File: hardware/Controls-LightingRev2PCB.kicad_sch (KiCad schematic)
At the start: 37 parts, among them IC2 AP2205-W5-7, IC3 ACS724LLCTR-05AU-T, IC4 ACS724LLCTR-05AU-T, IC6 ACS724LLCTR-05AU-T, J1 53307-2471, J3 Conn_02x05_Top_Bottom, J4 Conn_01x02, J5 Conn_01x02, J6 Conn_01x03, Q3 IRLML0030, Q5 IRLML0030, U5 SN74LV1T34DBV

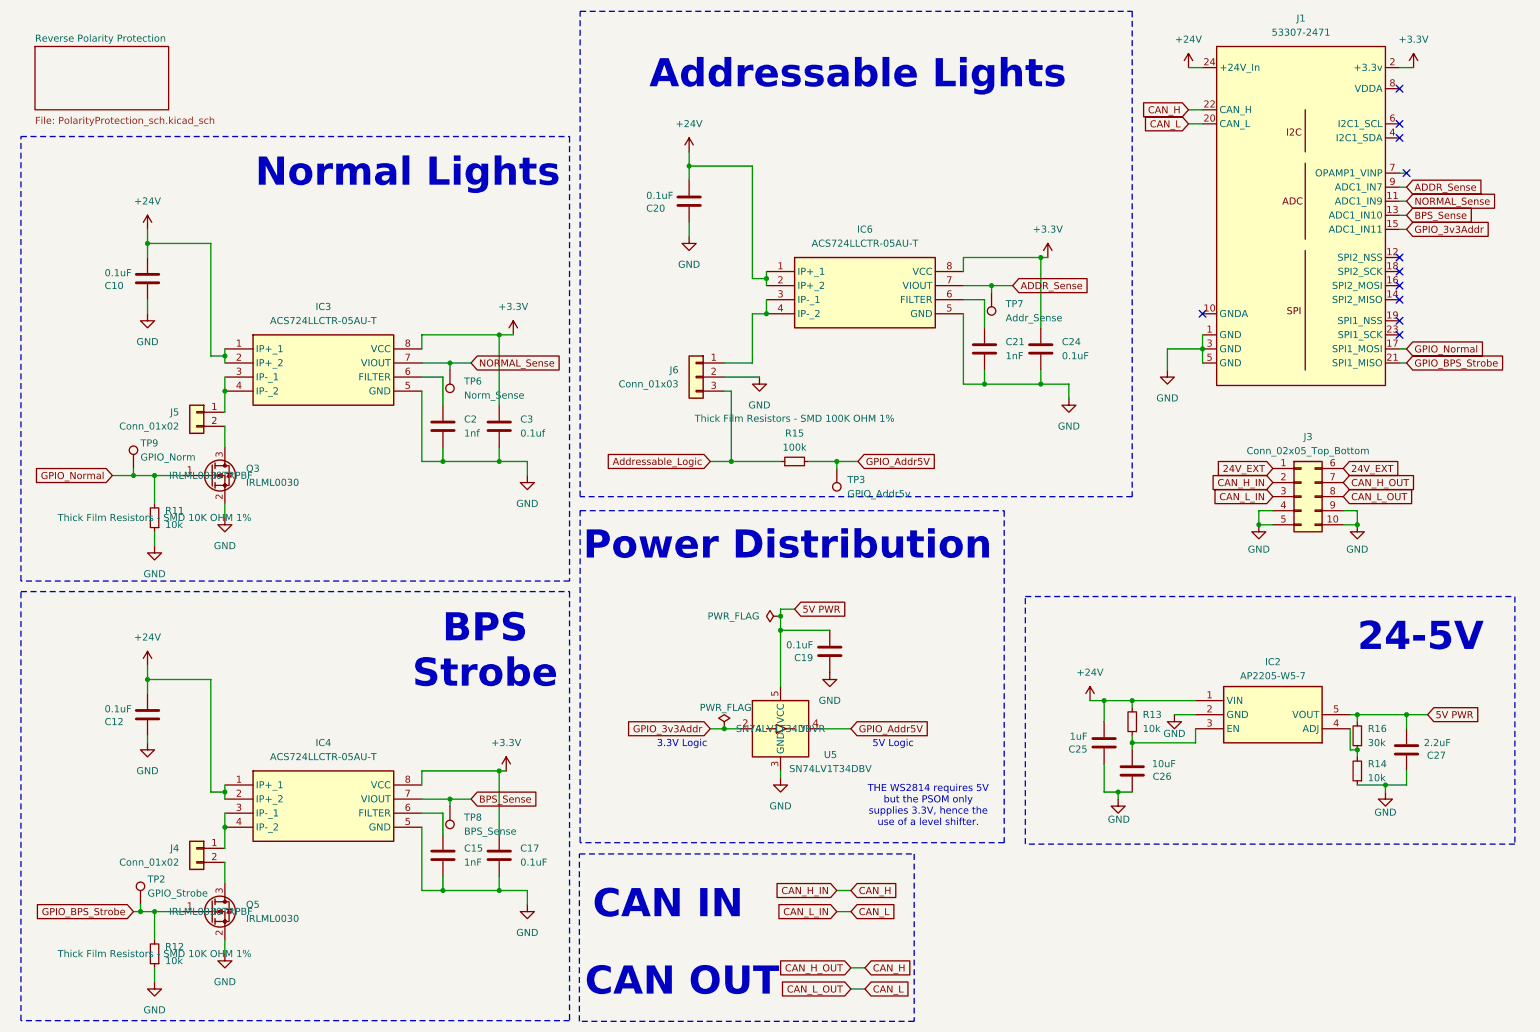
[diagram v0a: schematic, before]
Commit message: Bom and Final Layout
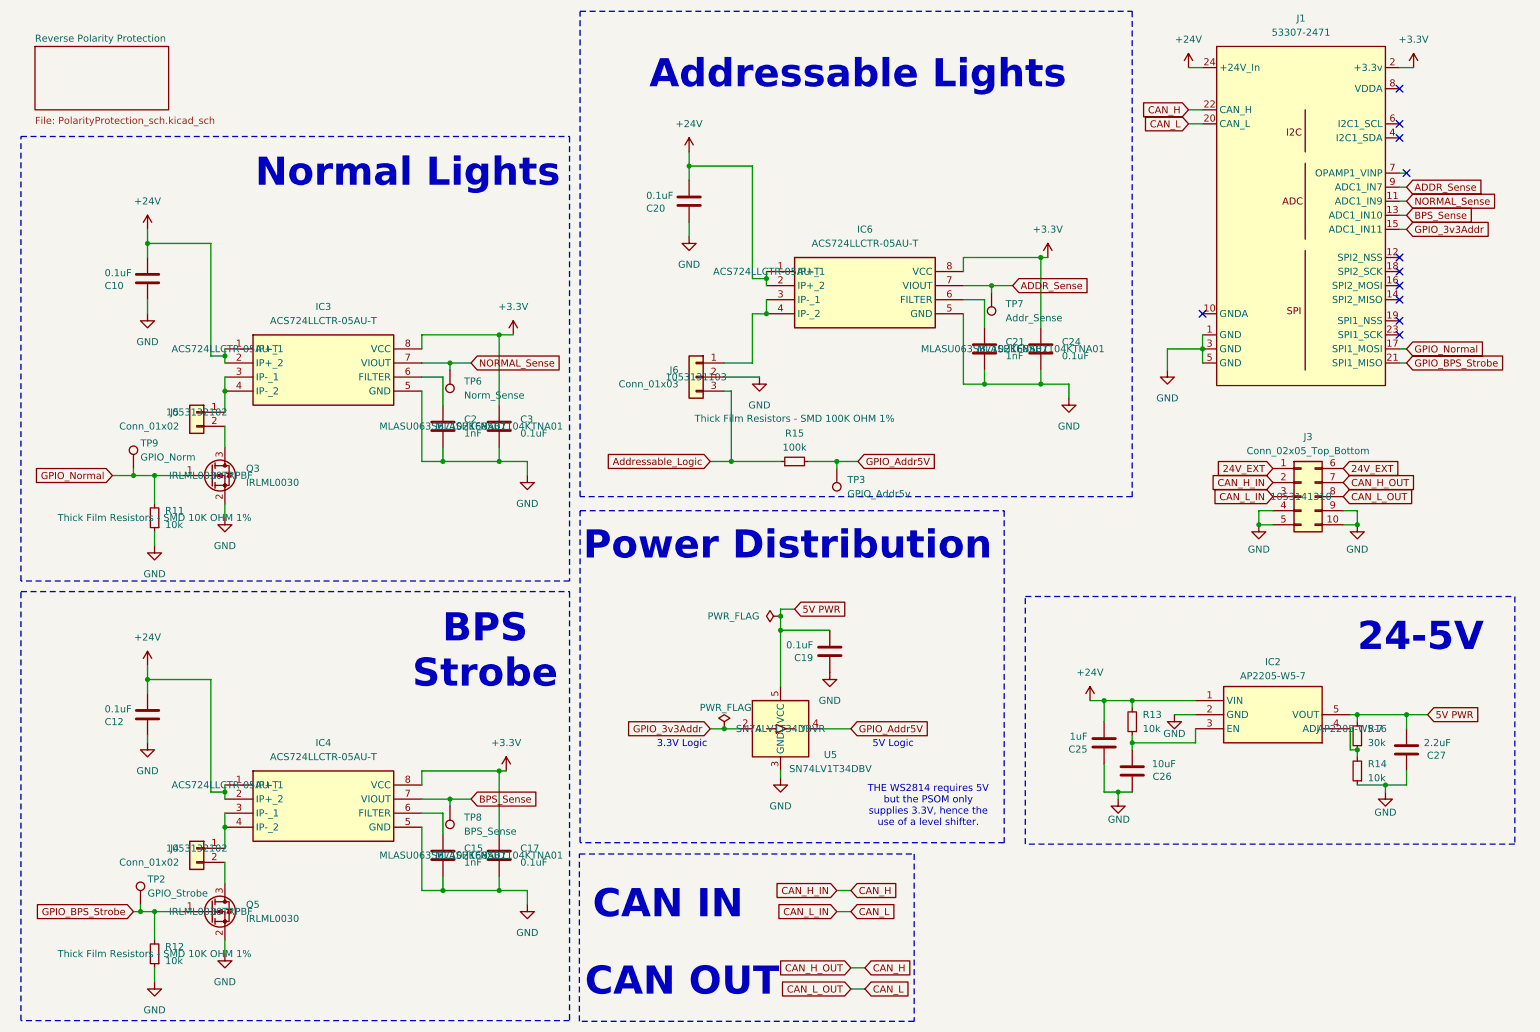
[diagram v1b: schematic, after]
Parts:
- C15, C21: P/N (none) -> MLASU063SB7102KFNA01
- C17, C24: P/N (none) -> MLASH168SB7104KTNA01
- C2: value 1nf -> 1nF; P/N (none) -> MLASU063SB7102KFNA01
- C26: P/N MLASH168SB7104KTNA01 -> GRM21BR61H106KE43K
- C27: P/N MLASH168SB7104KTNA01 -> GRT188R61H225KE13D
- C3: value 0.1uf -> 0.1uF; P/N (none) -> MLASH168SB7104KTNA01
- IC2: P/N (none) -> AP2205-W5-7
- IC3, IC4, IC6: P/N (none) -> ACS724LLCTR-05AU-T
- J3: P/N (none) -> 1053141310
- J4, J5: P/N (none) -> 1053132102
- J6: P/N (none) -> 1053131103
- R16: P/N CRCW060310K0FKEI -> CRCW060330K0FKEA
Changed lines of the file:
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@@
 			)
 		)
+		(property "P/N" "ACS724LLCTR-05AU-T"
+			(at 50.8 74.93 0)
+			(effects
+				(font
+					(size 1.27 1.27)
+				)
+			)
+		)
 		(pin "4"
 		)
@@
 			)
 		)
+		(property "P/N" "ACS724LLCTR-05AU-T"
+			(at 148.59 60.96 0)
+			(effects
+				(font
+					(size 1.27 1.27)
+				)
+			)
+		)
 		(pin "4"
 		)
@@
 			)
 		)
+		(property "P/N" "AP2205-W5-7 "
+			(at 254 143.51 0)
+			(effects
+				(font
+					(size 1.27 1.27)
+				)
+			)
+		)
 		(pin "5"
 		)
@@
 			)
 		)
+		(property "P/N" "1053132102"
+			(at 45.72 165.1 0)
+			(effects
+				(font
+					(size 1.27 1.27)
+				)
+			)
+		)
 		(pin "1"
 		)
@@
 			)
 		)
+		(property "P/N" "MLASU063SB7102KFNA01"
+			(at 90.17 166.37 0)
+			(effects
+				(font
+					(size 1.27 1.27)
+				)
+			)
+		)
 		(pin "2"
 		)
@@
 			)
 		)
-		(property "P/N" "MLASH168SB7104KTNA01"
+		(property "P/N" "GRM21BR61H106KE43K"
 			(at 214.63 151.13 0)
 			(effects
@@
 			)
 		)
+		(property "P/N" "MLASH168SB7104KTNA01"
+			(at 198.12 74.93 0)
+			(effects
+				(font
+					(size 1.27 1.27)
+				)
+			)
+		)
 		(pin "2"
 		)
@@
 			)
 		)
+		(property "P/N" "MLASU063SB7102KFNA01"
+			(at 187.96 74.93 0)
+			(effects
+				(font
+					(size 1.27 1.27)
+				)
+			)
+		)
 		(pin "2"
 		)
@@
 			)
 		)
-		(property "Value" "1nf"
+		(property "Value" "1nF"
 			(at 93.98 90.1699 0)
 			(effects
@@
 			)
 		)
+		(property "P/N" "MLASU063SB7102KFNA01"
+			(at 90.17 88.9 0)
+			(effects
+				(font
+					(size 1.27 1.27)
+				)
+			)
+		)
 		(pin "2"
 		)
@@
 			)
 		)
-		(property "P/N" "CRCW060310K0FKEI "
+		(property "P/N" "CRCW060330K0FKEA"
 			(at 255.27 144.78 0)
 			(effects
@@
 			)
 		)
+		(property "P/N" "MLASH168SB7104KTNA01"
+			(at 100.33 166.37 0)
+			(effects
+				(font
+					(size 1.27 1.27)
+				)
+			)
+		)
 		(pin "2"
 		)
@@
 			)
 		)
+		(property "P/N" "1053141310"
+			(at 245.11 101.6 0)
+			(effects
+				(font
+					(size 1.27 1.27)
+				)
+			)
+		)
 		(pin "2"
 		)
@@
 			)
 		)
-		(property "Value" "0.1uf"
+		(property "Value" "0.1uF"
 			(at 104.14 90.1699 0)
 			(effects
@@
 			)
 		)
+		(property "P/N" "MLASH168SB7104KTNA01"
+			(at 100.33 88.9 0)
+			(effects
+				(font
+					(size 1.27 1.27)
+				)
+			)
+		)
 		(pin "2"
 		)
@@
 			)
 		)
+		(property "P/N" "ACS724LLCTR-05AU-T"
+			(at 50.8 153.67 0)
+			(effects
+				(font
+					(size 1.27 1.27)
+				)
+			)
+		)
 		(pin "4"
 		)
@@
 			)
 		)
-		(property "P/N" "MLASH168SB7104KTNA01"
+		(property "P/N" "GRT188R61H225KE13D"
 			(at 264.16 147.32 0)
 			(effects
@@
 			)
 		)
+		(property "P/N" "1053131103 "
+			(at 135.89 80.01 0)
+			(effects
+				(font
+					(size 1.27 1.27)
+				)
+			)
+		)
 		(pin "1"
 		)
@@
 			)
 		)
+		(property "P/N" "1053132102"
+			(at 45.72 86.36 0)
+			(effects
+				(font
+					(size 1.27 1.27)
+				)
+			)
+		)
